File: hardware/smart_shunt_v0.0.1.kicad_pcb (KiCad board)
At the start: 2 copper layers, 63.8 x 34.3 mm, 48 parts, among them J1 SHUNT +, J2 SHUNT -, J3 VIn, J4 USB_C_Receptacle_USB2.0, J5 GND, SW1 SW_Push, SW2 SW_Push, U1 ESP32-C3-MINI-1, U4 INA226, U5 TPS562201

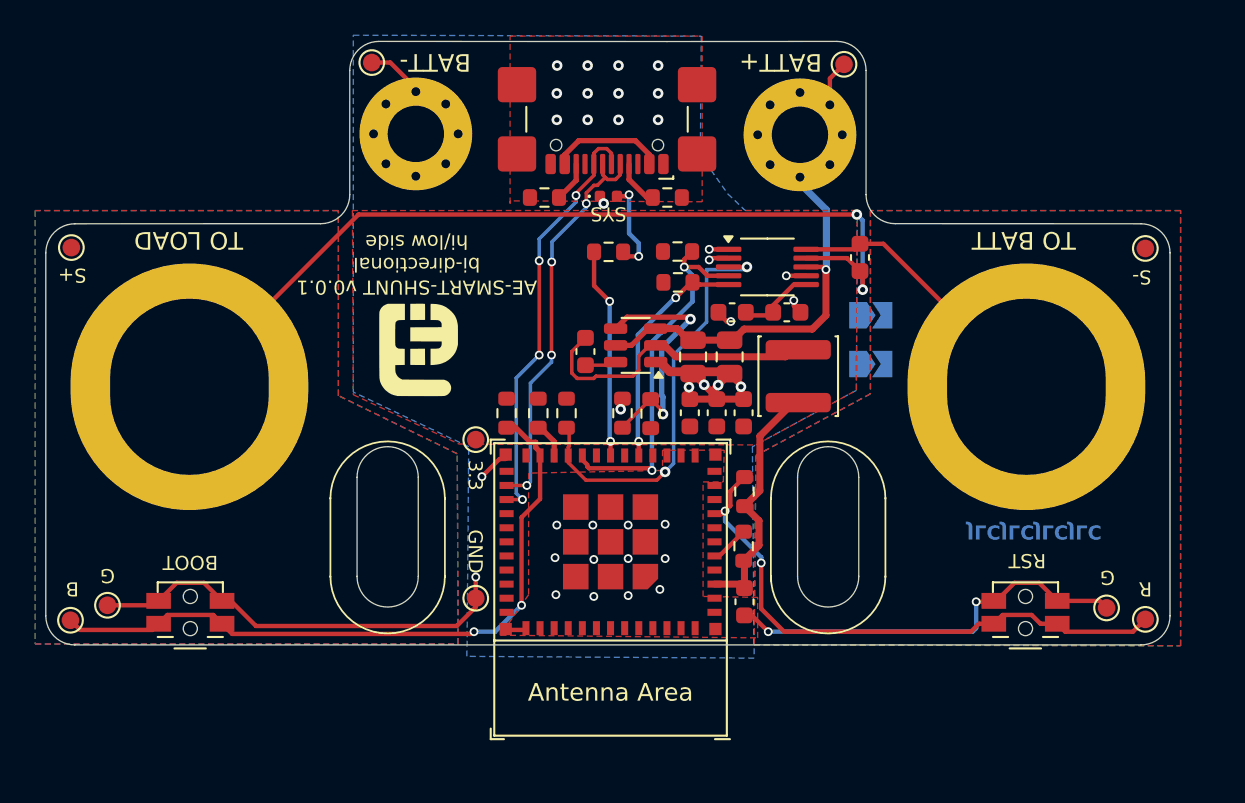
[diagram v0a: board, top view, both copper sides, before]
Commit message: v0.0.2 update, before FETs
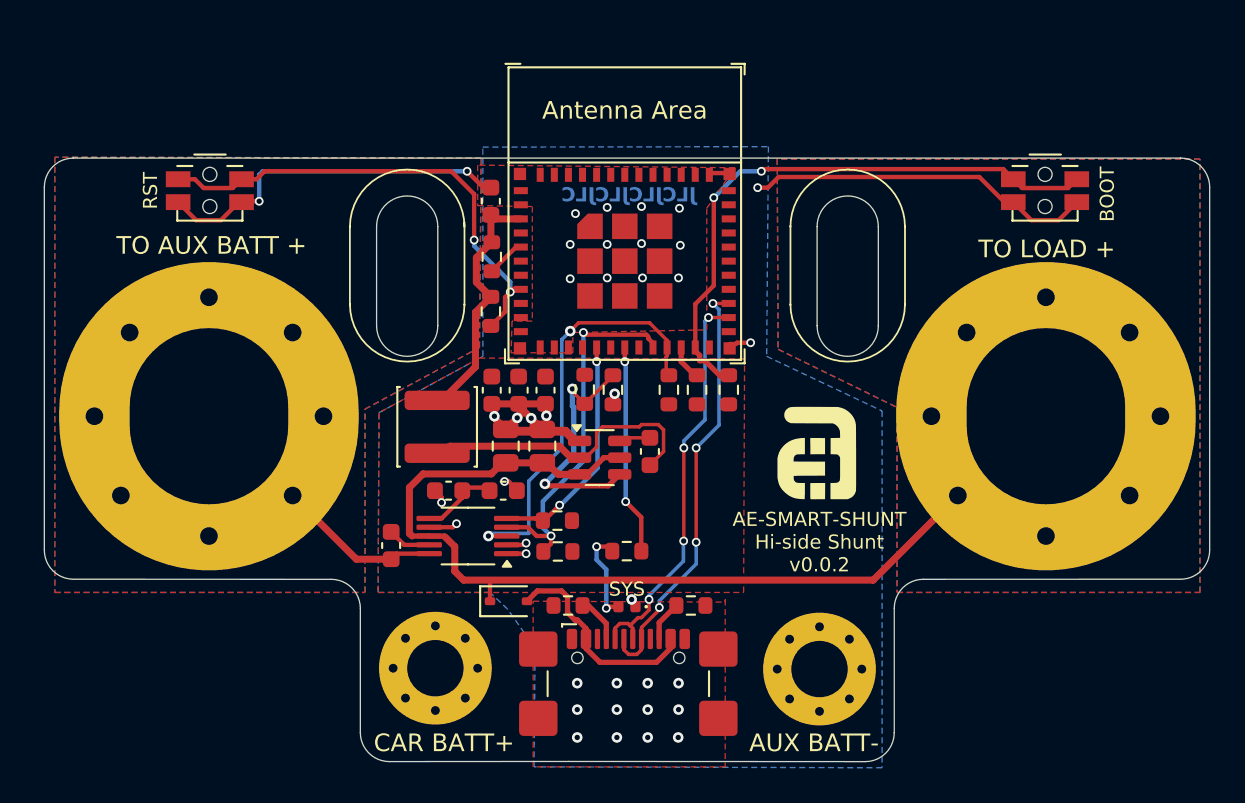
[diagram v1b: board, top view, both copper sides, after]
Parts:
- removed JP1 (x2): SolderJumper_2_Open, Jumper:SolderJumper-2_P1.3mm_Open_TrianglePad1.0x1.5mm
- removed TP3, TP4 (x4), TP5, TP6, TP7, TP8, TP9: TestPoint, TestPoint:TestPoint_Pad_D1.0mm
- added D5: 1N5819WS, Diode_SMD:D_SOD-323, F.Cu at (136.9, 92.2)
- J1, J2: footprint Acea:MountingHole_10.5mm -> ShuntToPCB:MountingHole_17mm
- moved SW2 54.1 mm to (167.3, 68.9), turned to 0 degrees
- moved SW1 52.1 mm to (119.9, 68.9), turned to 0 degrees
- moved J1 48.6 mm to (167.4, 81.7), turned to 180 degrees
- moved J2 46.4 mm to (119.9, 81.7), turned to 180 degrees
- moved J5 38.0 mm to (154.5, 96.0), turned to 180 degrees
- moved J3 36.7 mm to (132.7, 96.0), turned to 180 degrees
- moved J4 34.3 mm to (143.7, 98.0), turned to 0 degrees
- moved C8 31.2 mm to (130.2, 89.0), turned to 90 degrees
- moved C5 26.9 mm to (135.9, 69.5), turned to 90 degrees
- moved R10 24.6 mm to (147.2, 92.4), turned to 180 degrees
- moved R9 23.8 mm to (140.2, 92.4), turned to 0 degrees
- moved G*** 23.3 mm to (154.3, 83.8), turned to 0 degrees
- moved D1 23.3 mm to (143.6, 92.5), turned to 180 degrees
- moved U4 22.8 mm to (134.6, 88.5), turned to 180 degrees
- moved R6 21.8 mm to (135.9, 72.6), turned to -90 degrees
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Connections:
- C4 pad 1: BATTV -> SHUNT+
- C6 pad 1: BATTV -> SHUNT+
- J3 pad 1: BATTV -> unconnected-(J3-Pin_1-Pad1)
- U1 pad 19: unconnected-(U1-GPIO5/ADC2_CH0-Pad19) -> LOAD_DISCONNECT
- U4 pad 8: BATTV -> SHUNT+
- U5 pad 3: BATTV -> SHUNT+
- U5 pad 5: BATTV -> SHUNT+
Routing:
- net BATTV: track 24.6 -> 0.00 mm, vias 1 -> 0
- net GND: track 72.5 -> 61.8 mm
- net SHUNT-: track 16.0 -> 9.38 mm
- net USB_VBUS: track 6.52 -> 12.1 mm
- net Net-(U1-EN/CHIP_PU): track 32.9 -> 27.4 mm
- net Net-(U1-GPIO9): track 38.6 -> 33.2 mm
- net SHUNT+: track 50.5 -> 54.0 mm, vias 2 -> 0
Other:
- board size 63.8 x 34.3 mm -> 66.1 x 34.3 mm
- board text added: "AE-SMART-SHUNT Hi-side Shunt v0.0.2"
- board text added: "AUX BATT-"
- board text added: "CAR BATT+"
- board text added: "TO AUX BATT +"
- board text added: "TO LOAD +"
- board text removed: "3.3"
- board text removed: "AE-SMART-SHUNT v0.0.1 bi-directional hi/low side"
- board text removed: "B"
- board text removed: "BATT+"
- board text removed: "BATT-"
- board text removed: "G"
- board text removed: "GND"
- board text removed: "R"
- board text removed: "S+"
- board text removed: "S-"
- board text removed: "TO BATT"
- board text removed: "TO LOAD"
